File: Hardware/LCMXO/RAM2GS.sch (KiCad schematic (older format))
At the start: 63 parts, among them J1 Memory Expansion, J2 JTAG, U1 LCMXO256C-3TN100C, U10 74LVC1G04GW, U11 AP2127K-1.2TRG1, U12 25F010, U2 W9812G6KH-6, U3 60M, U4 74AHCT245PW, U5 74LVC245APW, U6 74LVC245APW, U7 74LVC245APW, U8 AZ1117CH-3.3TRG1, U9 74LVC1G04GW

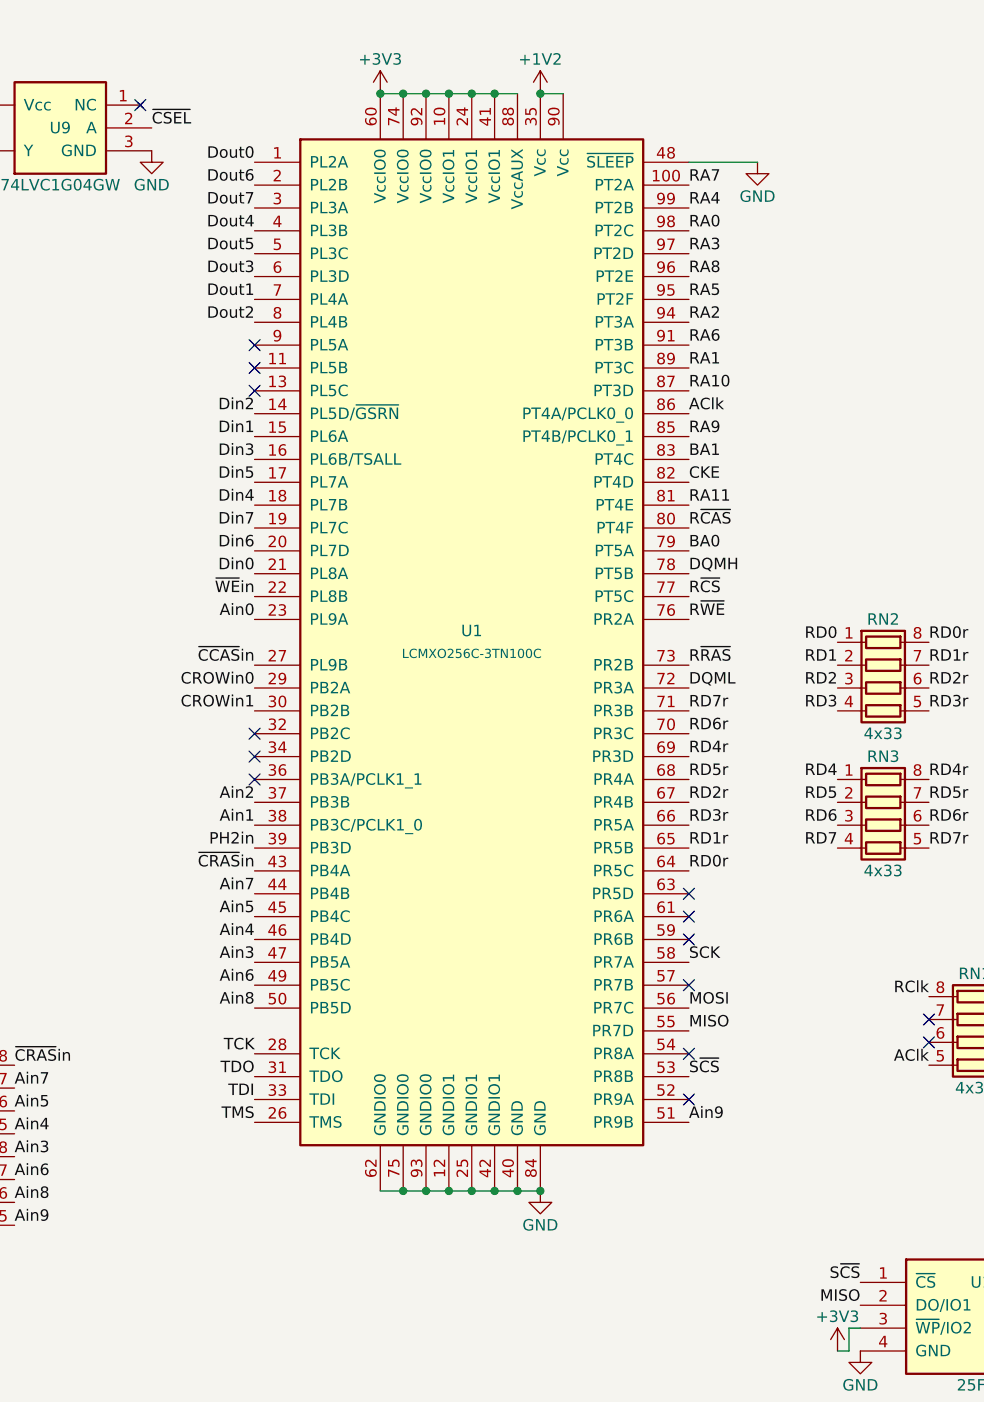
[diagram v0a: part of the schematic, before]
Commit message: more
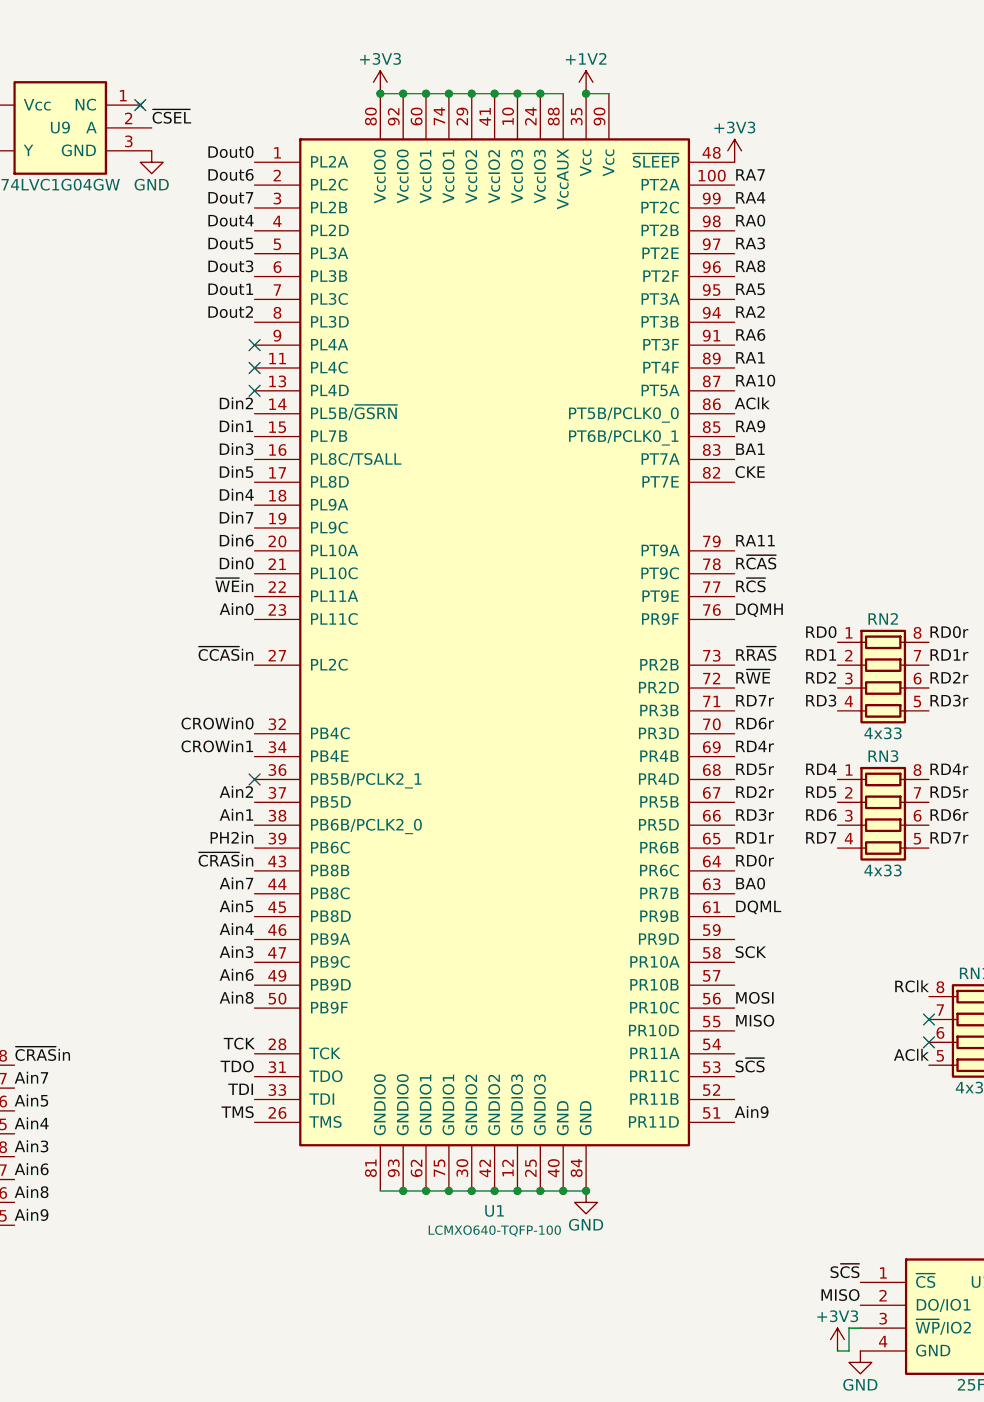
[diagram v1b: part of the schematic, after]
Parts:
- removed U1: LCMXO256C-3TN100C, stdpads:TQFP-100_14x14mm_P0.5mm, symbol GW_PLD:LCMXO256-TQFP-100
- added U1: LCMXO640-TQFP-100, stdpads:TQFP-100, symbol GW_PLD:LCMXO640-TQFP-100
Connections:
- net +1V2: now also U1.35 (Vcc), U1.90 (Vcc)
- net +3V3: now also U1.10 (VccIO3), U1.24 (VccIO3), U1.29 (VccIO2), U1.41 (VccIO2), U1.48 (~SLEEP~), U1.60 (VccIO1), U1.74 (VccIO1), U1.80 (VccIO0), U1.88 (VccAUX), U1.92 (VccIO0)
- net AClk: now also U1.86 (PT5B/PCLK0_0)
- net Ain0: now also U1.23 (PL11C)
- net Ain1: now also U1.38 (PB6B/PCLK2_0)
- net Ain2: now also U1.37 (PB5D)
- net Ain3: now also U1.47 (PB9C)
- net Ain4: now also U1.46 (PB9A)
- net Ain5: now also U1.45 (PB8D)
- net Ain6: now also U1.49 (PB9D)
- net Ain7: now also U1.44 (PB8C)
- net Ain8: now also U1.50 (PB9F)
- net Ain9: now also U1.51 (PR11D)
- net BA0: now also U1.63 (PR7B)
- net BA1: now also U1.83 (PT7A)
- net CKE: now also U1.82 (PT7E)
- net CROWin0: now also U1.32 (PB4C)
- net CROWin1: now also U1.34 (PB4E)
- net DQMH: now also U1.76 (PR9F)
- net DQML: now also U1.61 (PR9B)
- net Din0: now also U1.21 (PL10C)
- net Din1: now also U1.15 (PL7B)
- net Din2: now also U1.14 (PL5B/~GSRN~)
- net Din3: now also U1.16 (PL8C/TSALL)
- net Din4: now also U1.18 (PL9A)
- net Din5: now also U1.17 (PL8D)
- net Din6: now also U1.20 (PL10A)
- net Din7: now also U1.19 (PL9C)
- net Dout0: now also U1.1 (PL2A)
- net Dout1: now also U1.7 (PL3C)
- net Dout2: now also U1.8 (PL3D)
- net Dout3: now also U1.6 (PL3B)
- net Dout4: now also U1.4 (PL2D)
- net Dout5: now also U1.5 (PL3A)
- net Dout6: now also U1.2 (PL2C)
- net Dout7: now also U1.3 (PL2B)
- net GND: now also U1.12 (GNDIO3), U1.25 (GNDIO3), U1.30 (GNDIO2), U1.40 (GND), U1.42 (GNDIO2), U1.62 (GNDIO1), U1.75 (GNDIO1), U1.81 (GNDIO0), U1.84 (GND), U1.93 (GNDIO0)
- net MISO: now also U1.55 (PR10D)
- net MOSI: now also U1.56 (PR10C)
- net PH2in: now also U1.39 (PB6C)
- net RA0: now also U1.98 (PT2B)
- net RA1: now also U1.89 (PT4F)
- net RA10: now also U1.87 (PT5A)
- net RA11: now also U1.79 (PT9A)
- net RA2: now also U1.94 (PT3B)
- net RA3: now also U1.97 (PT2E)
- net RA4: now also U1.99 (PT2C)
- net RA5: now also U1.95 (PT3A)
- net RA6: now also U1.91 (PT3F)
- net RA7: now also U1.100 (PT2A)
- net RA8: now also U1.96 (PT2F)
- net RA9: now also U1.85 (PT6B/PCLK0_1)
- net RD0r: now also U1.64 (PR6C)
- net RD1r: now also U1.65 (PR6B)
- net RD2r: now also U1.67 (PR5B)
- net RD3r: now also U1.66 (PR5D)
- net RD4r: now also U1.69 (PR4B)
- net RD5r: now also U1.68 (PR4D)
- net RD6r: now also U1.70 (PR3D)
- net RD7r: now also U1.71 (PR3B)
- net R~CAS~: now also U1.78 (PT9C)
- net R~CS~: now also U1.77 (PT9E)
- net R~RAS~: now also U1.73 (PR2B)
- net R~WE~: now also U1.72 (PR2D)
- net SCK: now also U1.58 (PR10A)
- net S~CS~: now also U1.53 (PR11C)
- net TCK: now also U1.28 (TCK)
- net TDI: now also U1.33 (TDI)
- net TDO: now also U1.31 (TDO)
- net TMS: now also U1.26 (TMS)
- net ~CCAS~in: now also U1.27 (PL2C)
- net ~CRAS~in: now also U1.43 (PB8B)
- net ~WE~in: now also U1.22 (PL11A)
- no-connect marks 22 -> 14
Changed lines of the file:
@@
 Text Label 8900 3900 2    50   ~ 0
 RClk
-Text Label 7250 2300 0    50   ~ 0
+Text Label 7450 2300 0    50   ~ 0
 AClk
 Wire Wire Line
@@
 L power:GND #PWR0136
 U 1 1 5E9DF65F
-P 6600 5700
-F 0 "#PWR0136" H 6600 5450 50  0001 C CNN
-F 1 "GND" H 6600 5550 50  0000 C CNN
-F 2 "" H 6600 5700 50  0001 C CNN
-F 3 "" H 6600 5700 50  0001 C CNN
-	1    6600 5700
+P 6800 5700
+F 0 "#PWR0136" H 6800 5450 50  0001 C CNN
+F 1 "GND" H 6800 5550 50  0000 C CNN
+F 2 "" H 6800 5700 50  0001 C CNN
+F 3 "" H 6800 5700 50  0001 C CNN
+	1    6800 5700
 	-1   0    0    -1
 $EndComp
@@
 Text Label 5350 3200 2    50   ~ 0
 Ain0
-Text Label 5350 3600 2    50   ~ 0
+Text Label 5350 3800 2    50   ~ 0
 CROWin1
-Text Label 5350 3500 2    50   ~ 0
+Text Label 5350 3700 2    50   ~ 0
 CROWin0
 Text Label 5350 3400 2    50   ~ 0
@@
 Text Label 5350 4900 2    50   ~ 0
 Ain8
-Text Label 7250 3000 0    50   ~ 0
+Text Label 7450 3200 0    50   ~ 0
 DQMH
-Text Label 7250 2800 0    50   ~ 0
+Text Label 7450 3000 0    50   ~ 0
 R~CAS~
-Text Label 7250 2600 0    50   ~ 0
+Text Label 7450 2600 0    50   ~ 0
 CKE
-Text Label 7250 3400 0    50   ~ 0
+Text Label 7450 3400 0    50   ~ 0
 R~RAS~
-Text Label 7250 3100 0    50   ~ 0
+Text Label 7450 3100 0    50   ~ 0
 R~CS~
-Text Label 7250 2900 0    50   ~ 0
+Text Label 7450 4400 0    50   ~ 0
 BA0
-Text Label 7250 2700 0    50   ~ 0
+Text Label 7450 2900 0    50   ~ 0
 RA11
-Text Label 7250 2500 0    50   ~ 0
+Text Label 7450 2500 0    50   ~ 0
 BA1
-Text Label 7250 2400 0    50   ~ 0
+Text Label 7450 2400 0    50   ~ 0
 RA9
-Text Label 7250 2200 0    50   ~ 0
+Text Label 7450 2200 0    50   ~ 0
 RA10
-Text Label 7250 1700 0    50   ~ 0
+Text Label 7450 1700 0    50   ~ 0
 RA8
-Text Label 7250 1500 0    50   ~ 0
+Text Label 7450 1500 0    50   ~ 0
 RA0
-Text Label 7250 1300 0    50   ~ 0
+Text Label 7450 1300 0    50   ~ 0
 RA7
-Text Label 7250 2100 0    50   ~ 0
+Text Label 7450 2100 0    50   ~ 0
 RA1
-Text Label 7250 2000 0    50   ~ 0
+Text Label 7450 2000 0    50   ~ 0
 RA6
-Text Label 7250 1900 0    50   ~ 0
+Text Label 7450 1900 0    50   ~ 0
 RA2
-Text Label 7250 1600 0    50   ~ 0
+Text Label 7450 1600 0    50   ~ 0
 RA3
-Text Label 7250 1400 0    50   ~ 0
+Text Label 7450 1400 0    50   ~ 0
 RA4
-Text Label 7250 1800 0    50   ~ 0
+Text Label 7450 1800 0    50   ~ 0
 RA5
 $Comp
@@
 	0    1    -1   0
 $EndComp
-Text Label 7250 5200 0    50   ~ 0
+Text Label 7450 5200 0    50   ~ 0
 S~CS~
-Text Label 7250 4700 0    50   ~ 0
+Text Label 7450 4700 0    50   ~ 0
 SCK
-Text Label 7250 4900 0    50   ~ 0
+Text Label 7450 4900 0    50   ~ 0
 MOSI
-Text Label 7250 5000 0    50   ~ 0
+Text Label 7450 5000 0    50   ~ 0
 MISO
 Text Label 5350 4100 2    50   ~ 0
@@
 Text Label 5350 4000 2    50   ~ 0
 Ain2
-Text Label 7250 3200 0    50   ~ 0
+Text Label 7450 3500 0    50   ~ 0
 R~WE~
-Text Label 7250 3500 0    50   ~ 0
+Text Label 7450 4500 0    50   ~ 0
 DQML
-Text Label 7250 4300 0    50   ~ 0
+Text Label 7450 4300 0    50   ~ 0
 RD0r
-Text Label 7250 3600 0    50   ~ 0
+Text Label 7450 3600 0    50   ~ 0
 RD7r
-Text Label 7250 3700 0    50   ~ 0
+Text Label 7450 3700 0    50   ~ 0
 RD6r
-Text Label 7250 3900 0    50   ~ 0
+Text Label 7450 3900 0    50   ~ 0
 RD5r
-Text Label 7250 3800 0    50   ~ 0
+Text Label 7450 3800 0    50   ~ 0
 RD4r
-Text Label 7250 4100 0    50   ~ 0
+Text Label 7450 4100 0    50   ~ 0
 RD3r
-Text Label 7250 4000 0    50   ~ 0
+Text Label 7450 4000 0    50   ~ 0
 RD2r
-Text Label 7250 4200 0    50   ~ 0
+Text Label 7450 4200 0    50   ~ 0
 RD1r
 Text Label 5350 5400 2    50   ~ 0
@@
 $EndComp
 Connection ~ 2250 6750
-Text Label 7250 5400 0    50   ~ 0
+Text Label 7450 5400 0    50   ~ 0
 Ain9
-Connection ~ 6200 5700
-Connection ~ 6600 5700
-Connection ~ 6400 5700
-Connection ~ 6200 900
-Wire Wire Line
-	6300 5700 6400 5700
-Wire Wire Line
-	6200 5700 6300 5700
-Connection ~ 6300 5700
-Wire Wire Line
-	6300 900  6400 900
-Wire Wire Line
-	6200 900  6300 900
-Connection ~ 6300 900
-Wire Wire Line
-	6100 5700 6200 5700
-Connection ~ 6100 5700
-Wire Wire Line
-	6100 900  6200 900
-Connection ~ 6100 900
-Wire Wire Line
-	6500 5700 6600 5700
-Wire Wire Line
-	6400 5700 6500 5700
-Connection ~ 6500 5700
 Wire Wire Line
 	6600 900  6700 900
-Wire Wire Line
-	6000 900  6100 900
-Wire Wire Line
-	5900 900  6000 900
-Connection ~ 6000 900
-Wire Wire Line
-	6000 5700 6100 5700
-Wire Wire Line
-	5900 5700 6000 5700
-Connection ~ 6000 5700
-Connection ~ 5900 900
 Wire Wire Line
 	4000 6950 4000 7050
 Connection ~ 4000 6950
-Connection ~ 6400 900
-Wire Wire Line
-	6400 900  6500 900
 $Comp
 L power:+1V2 #PWR0150
 U 1 1 8715E9C7
-P 6600 900
-F 0 "#PWR0150" H 6600 750 50  0001 C CNN
-F 1 "+1V2" H 6600 1050 50  0000 C CNN
-F 2 "" H 6600 900 50  0001 C CNN
-F 3 "" H 6600 900 50  0001 C CNN
-	1    6600 900
-	1    0    0    -1
-$EndComp
-Connection ~ 6600 900
+P 6800 900
+F 0 "#PWR0150" H 6800 750 50  0001 C CNN
+F 1 "+1V2" H 6800 1050 50  0000 C CNN
+F 2 "" H 6800 900 50  0001 C CNN
+F 3 "" H 6800 900 50  0001 C CNN
+	1    6800 900
+	1    0    0    -1
+$EndComp
 Wire Wire Line
 	1450 6950 1850 6950
@@
 	0    1    1    0
 $EndComp
-$Comp
-L GW_PLD:LCMXO256-TQFP-100 U1
-U 1 1 86DF1B11
-P 6300 3300
-F 0 "U1" H 6300 3350 50  0000 C CNN
-F 1 "LCMXO256C-3TN100C" H 6300 3250 40  0000 C CNN
-F 2 "stdpads:TQFP-100_14x14mm_P0.5mm" H 6300 3200 40  0001 C CNN
-F 3 "" H 6300 3400 50  0001 C CNN
-F 4 "C1521848" H 6300 3300 50  0001 C CNN "LCSC Part"
-F 5 "Lattice LCMXO256C-3TN100C, Lattice LCMXO256C-4TN100C, Lattice LCMXO256C-5TN100C" H 6300 3300 50  0001 C CNN "Mfg. Part Numbers"
-	1    6300 3300
-	1    0    0    -1
-$EndComp
 NoConn ~ 5350 2000
 NoConn ~ 5350 2100
 NoConn ~ 5350 2200
-NoConn ~ 5350 3700
-NoConn ~ 5350 3800
 NoConn ~ 5350 3900
-NoConn ~ 7250 4400
-NoConn ~ 7250 4500
-NoConn ~ 7250 4600
-NoConn ~ 7250 4800
-NoConn ~ 7250 5100
-NoConn ~ 7250 5300
 Wire Wire Line
 	1950 4300 1950 4550
@@
 	1950 3850 1850 3850
 $Comp
-L power:GND #PWR?
-U 1 1 60E703CE
-P 7550 1200
-F 0 "#PWR?" H 7550 950 50  0001 C CNN
-F 1 "GND" H 7550 1050 50  0000 C CNN
-F 2 "" H 7550 1200 50  0001 C CNN
-F 3 "" H 7550 1200 50  0001 C CNN
-	1    7550 1200
-	-1   0    0    -1
-$EndComp
-Wire Wire Line
-	7550 1200 7250 1200
+L power:+3V3 #PWR0168
+U 1 1 626AF4E6
+P 7450 1200
+F 0 "#PWR0168" H 7450 1050 50  0001 C CNN
+F 1 "+3V3" H 7450 1350 50  0000 C CNN
+F 2 "" H 7450 1200 50  0001 C CNN
+F 3 "" H 7450 1200 50  0001 C CNN
+	1    7450 1200
+	1    0    0    -1
+$EndComp
+Wire Wire Line
+	5900 900  6000 900
+Wire Wire Line
+	5900 5700 6000 5700
+$Comp
+L GW_PLD:LCMXO640-TQFP-100 U1
+U 1 1 62C26D47
+P 6400 3300
+F 0 "U1" H 6400 811 50  0000 C CNN
+F 1 "LCMXO640-TQFP-100" H 6400 727 40  0000 C CNN
+F 2 "stdpads:TQFP-100" H 6400 3200 40  0001 C CNN
+F 3 "" H 6400 3400 50  0001 C CNN
+	1    6400 3300
+	1    0    0    -1
+$EndComp
+Connection ~ 5900 900
+Wire Wire Line
+	6800 5700 6700 5700
+Connection ~ 6800 5700
+Connection ~ 6000 5700
+Connection ~ 6100 5700
+Wire Wire Line
+	6100 5700 6000 5700
+Connection ~ 6200 5700
+Wire Wire Line
+	6200 5700 6100 5700
+Connection ~ 6300 5700
+Wire Wire Line
+	6300 5700 6200 5700
+Connection ~ 6400 5700
+Wire Wire Line
+	6400 5700 6300 5700
+Connection ~ 6500 5700
+Wire Wire Line
+	6500 5700 6400 5700
+Connection ~ 6600 5700
+Wire Wire Line
+	6600 5700 6500 5700
+Connection ~ 6700 5700
+Wire Wire Line
+	6700 5700 6600 5700
+Wire Wire Line
+	6500 900  6400 900
+Connection ~ 6000 900
+Connection ~ 6100 900
+Wire Wire Line
+	6100 900  6000 900
+Connection ~ 6200 900
+Wire Wire Line
+	6200 900  6100 900
+Connection ~ 6300 900
+Wire Wire Line
+	6300 900  6200 900
+Connection ~ 6400 900
+Wire Wire Line
+	6400 900  6300 900
+Wire Wire Line
+	6600 900  6500 900
+Connection ~ 6600 900
+Connection ~ 6500 900
+Wire Wire Line
+	6800 900  6900 900
+Connection ~ 6800 900
 $EndSCHEMATC
